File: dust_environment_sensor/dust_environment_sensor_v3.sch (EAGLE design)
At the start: 49 parts, among them IC2 ATMEGA644A, J1 3.6V Lithium C cell, J2 EXP, J3 XBEE_1-10SMT, J4 XBEE_11-20SMT, U1 TSL2560T, U2 LIS3DH, U3 SI7005, U4 TSL2560CL, U5 AMN41121, U6 L3GD20, U7 MCP1700-3.3V, X2 32.768KHz

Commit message: tiny DES3
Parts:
- removed C13, C15, C5: 100n, rcl:C-EUC0603
- removed C14: 10u, rcl:C-USC0603
- removed C7: 4.7u, rcl:C-USC0603
- removed J2: EXP, SparkFun-Connectors:AVR_SPI_PRG_6PTH
- removed JP4, JP5, JP6, JP7: M01PTH, SparkFun-Connectors:M01PTH
- removed R3: 15, resistor:R-US_R0603
- removed U3: SI7005, Cool_Electricity:SI7005
- removed U6: L3GD20, Cool_Electricity:L3GD20
- added EXP: M05X2SHD, SparkFun-Connectors:M05X2SHD
- C4: value 100u -> 100n; device SparkFun-Capacitors:CAP_POL1206-KIT -> rcl:C-EUC0603
- JP9: device SparkFun-Connectors:M05X2PTH -> SparkFun-Connectors:M05X2SHD
- U4: value TSL2560CL -> HTU21D; device Cool_Electricity:TSL2560CL -> Cool_Electricity:HTU21D
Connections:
- removed net N$1: C7.1, U3.CEXT
- removed net N$11: C5.1, R3.2, U3.VDD
- removed net N$2: C15.1, U6.CAP
- new net MOTE_ASSOCIATED: J4.ON/!SLEEP
- new net MOTE_CONNECT: J3.PWM0/RSSI
- new net MOTE_SLEEP: J3.DIO12
- new net MOTE_TCPSTATUS: J4.ASSOC/AD5/DIO5
- net EXP_CSN: now also EXP.9; no longer J2.5
- net EXP_MISO: now also EXP.5; no longer J2.1
- net EXP_MOSI: now also EXP.8; no longer J2.4
- net EXP_SCK: now also EXP.7; no longer J2.3
- net GND: now also C4.2, EXP.10, EXP.4; no longer C13.2, C14.2, C15.2, C4.-, C5.2, C7.2, J2.6, JP4.1, JP5.1, JP6.1, JP7.1, U3.GND@1, U3.GND@2, U3.GND@3, U3.GND@4, U3.PAD, U4.ADDR, U6.GND, U6.RES/GND@1, U6.RES/GND@2, U6.RES/GND@3, U6.RES/GND@4, U6.RES/GND@5
- net GYRO_INT2: no longer U6.DRDY/INT2
- net HUMID_CS: no longer U3.#CS
- net HUMID_VCC: no longer R3.1
- net I2C_SCL: now also EXP.2; no longer U3.SCL, U6.SCL/SPC
- net I2C_SDA: now also EXP.1; no longer U3.SDA, U6.SDA/SDI/SDO
- net LIGHT_INT: no longer U4.INT
- net MOTE_ASSOC: no longer J4.ASSOC/AD5/DIO5
- net MOTE_STATUS: no longer J4.ON/!SLEEP
- net VBATT: now also EXP.6; no longer C4.+, J2.2
- net VCC: now also C4.1, EXP.3; no longer C13.1, C14.1, U6.CS, U6.RES/VDD, U6.SDO/SA0, U6.VDD, U6.VDD_IO
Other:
- note added: "1: VCC 2: UART_TX 3: UART_RX 4: GPIO 8 / TRIGSLP 5: RESET 6: GPIO 5 / TRIGTCP / LED 7: GPIO 7 8: GPIO 9 9: GPIO 1 10: GND"
- note added: "20: SEN 2 19: GPIO 2 18: GPIO 3 17: SEN 5 16: UART_CTS 15: GPIO 6/ TCPSTATUS / LED 14: NC 13: GPIO4/ ASSOC / LED 12: UART_RTS 11: GPIO 14"
- note added: "Wifly Pinout"
- note removed: "I2C ADDRESS: 10000000"

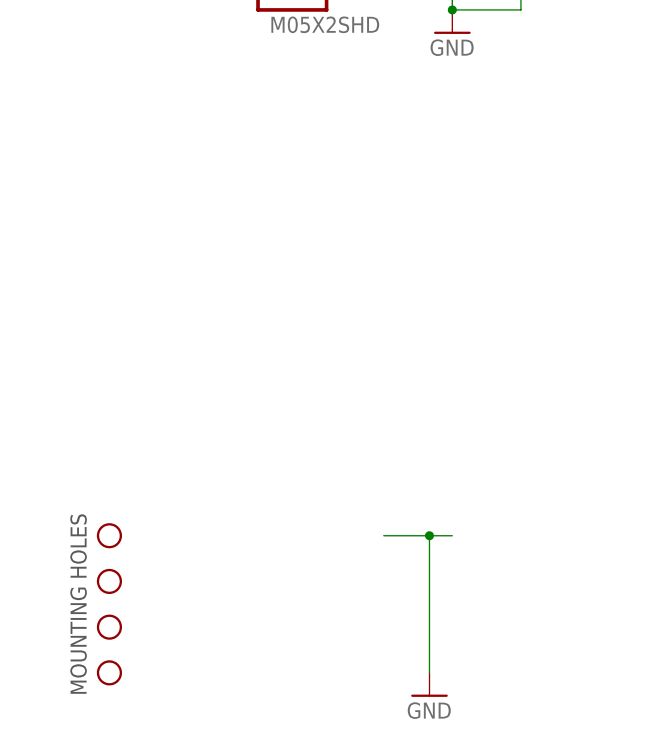
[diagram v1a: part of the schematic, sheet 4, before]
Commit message: schematic and placement done?
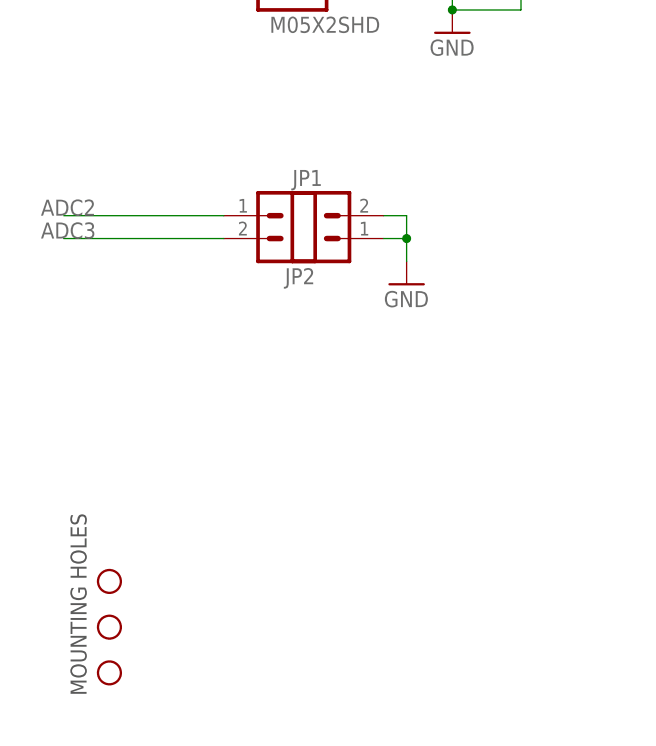
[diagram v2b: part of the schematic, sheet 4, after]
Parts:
- removed STANDOFF4: STAND-OFF, SparkFun-Electromechanical:STAND-OFF
- added JP1, JP2: (no value), SparkFun-Connectors:M02PTH
- J1: device Cool_Electricity:BX0036 -> Cool_Electricity:BX0036NH
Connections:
- removed net GYRO_INT2: IC2.(PCINT11/OC0A/AIN1)PB3
- removed net HUMID_CS: IC2.(PCINT2/ADC2)PA2
- removed net HUMID_VCC: IC2.(PCINT3/ADC3)PA3
- removed net MOTE_ASSOC: IC2.(PCINT9/CLKO/T1)PB1
- removed net MOTE_SLEEPN: IC2.(PCINT5/ADC5)PA5, J3.!DTR!/SLEEP_RQ/DIO8
- removed net MOTE_STATUS: IC2.(PCINT10/INT2/AIN0)PB2
- new net ADC2: IC2.(PCINT2/ADC2)PA2, JP2.1
- new net ADC3: IC2.(PCINT3/ADC3)PA3, JP2.2
- net GND: now also JP1.1, JP1.2
- net MOTE_ASSOCIATED: now also IC2.(PCINT11/OC0A/AIN1)PB3
- net MOTE_CONNECT: now also IC2.(PCINT9/CLKO/T1)PB1
- net MOTE_SLEEP: now also IC2.(PCINT5/ADC5)PA5
- net MOTE_TCPSTATUS: now also IC2.(PCINT10/INT2/AIN0)PB2
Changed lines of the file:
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@@
 <part name="GND2" library="supply1" deviceset="GND" device=""/>
 <part name="GND6" library="supply1" deviceset="GND" device=""/>
-<part name="J1" library="Cool_Electricity" deviceset="BX0036" device="" value="3.6V Lithium C cell"/>
+<part name="J1" library="Cool_Electricity" deviceset="BX0036" device="NH" value="3.6V Lithium C cell"/>
 <part name="GND7" library="supply1" deviceset="GND" device=""/>
 <part name="P+2" library="supply1" deviceset="VCC" device=""/>
@@
 <part name="STANDOFF2" library="SparkFun-Electromechanical" deviceset="STAND-OFF" device=""/>
 <part name="STANDOFF3" library="SparkFun-Electromechanical" deviceset="STAND-OFF" device=""/>
-<part name="STANDOFF4" library="SparkFun-Electromechanical" deviceset="STAND-OFF" device=""/>
-<part name="GND16" library="supply1" deviceset="GND" device=""/>
 <part name="GND17" library="SparkFun" deviceset="GND" device=""/>
 <part name="C8" library="rcl" deviceset="C-EU" device="C0603" value="100n"/>
@@
 <part name="GND13" library="supply1" deviceset="GND" device=""/>
 <part name="P+8" library="supply1" deviceset="VCC" device=""/>
+<part name="JP1" library="SparkFun-Connectors" deviceset="M02" device="PTH"/>
+<part name="JP2" library="SparkFun-Connectors" deviceset="M02" device="PTH"/>
+<part name="GND3" library="SparkFun" deviceset="GND" device=""/>
 </parts>
 <sheets>
@@
 <pinref part="IC2" gate="G$1" pin="(PCINT6/ADC6)PA6"/>
 <wire x1="119.38" y1="106.68" x2="160.02" y2="106.68" width="0.1524" layer="91"/>
-<label x="147.32" y="106.68" size="1.778" layer="95"/>
+<label x="142.24" y="106.68" size="1.778" layer="95"/>
 </segment>
 </net>
@@
 <wire x1="119.38" y1="38.1" x2="160.02" y2="38.1" width="0.1524" layer="91"/>
 <label x="134.62" y="38.1" size="1.778" layer="95"/>
-</segment>
-</net>
-<net name="MOTE_SLEEPN" class="0">
-<segment>
-<pinref part="IC2" gate="G$1" pin="(PCINT5/ADC5)PA5"/>
-<wire x1="119.38" y1="104.14" x2="160.02" y2="104.14" width="0.1524" layer="91"/>
-<label x="142.24" y="104.14" size="1.778" layer="95"/>
 </segment>
 </net>
@@
 </segment>
 </net>
-<net name="GYRO_INT2" class="0">
-<segment>
-<pinref part="IC2" gate="G$1" pin="(PCINT11/OC0A/AIN1)PB3"/>
-<wire x1="119.38" y1="76.2" x2="154.94" y2="76.2" width="0.1524" layer="91"/>
-<label x="144.78" y="76.2" size="1.778" layer="95"/>
-</segment>
-</net>
-<net name="HUMID_CS" class="0">
-<segment>
-<pinref part="IC2" gate="G$1" pin="(PCINT2/ADC2)PA2"/>
-<wire x1="119.38" y1="96.52" x2="157.48" y2="96.52" width="0.1524" layer="91"/>
-<label x="137.16" y="96.52" size="1.778" layer="95"/>
-</segment>
-</net>
-<net name="HUMID_VCC" class="0">
-<segment>
-<pinref part="IC2" gate="G$1" pin="(PCINT3/ADC3)PA3"/>
-<wire x1="119.38" y1="99.06" x2="160.02" y2="99.06" width="0.1524" layer="91"/>
-<label x="139.7" y="99.06" size="1.778" layer="95"/>
-</segment>
-</net>
-<net name="MOTE_STATUS" class="0">
+<net name="MOTE_TCPSTATUS" class="0">
 <segment>
 <pinref part="IC2" gate="G$1" pin="(PCINT10/INT2/AIN0)PB2"/>
@@
 </segment>
 </net>
-<net name="MOTE_ASSOC" class="0">
+<net name="MOTE_TX_CTSN" class="0">
+<segment>
+<pinref part="IC2" gate="G$1" pin="(PCINT8/XCK0/T0)PB0"/>
+<wire x1="119.38" y1="68.58" x2="152.4" y2="68.58" width="0.1524" layer="91"/>
+<label x="139.7" y="68.58" size="1.778" layer="95"/>
+</segment>
+</net>
+<net name="MOTE_CONNECT" class="0">
 <segment>
 <pinref part="IC2" gate="G$1" pin="(PCINT9/CLKO/T1)PB1"/>
@@
 </segment>
 </net>
-<net name="MOTE_TX_CTSN" class="0">
-<segment>
-<pinref part="IC2" gate="G$1" pin="(PCINT8/XCK0/T0)PB0"/>
-<wire x1="119.38" y1="68.58" x2="152.4" y2="68.58" width="0.1524" layer="91"/>
-<label x="139.7" y="68.58" size="1.778" layer="95"/>
+<net name="ADC2" class="0">
+<segment>
+<pinref part="IC2" gate="G$1" pin="(PCINT2/ADC2)PA2"/>
+<wire x1="119.38" y1="96.52" x2="157.48" y2="96.52" width="0.1524" layer="91"/>
+<label x="142.24" y="96.52" size="1.778" layer="95"/>
+</segment>
+</net>
+<net name="MOTE_ASSOCIATED" class="0">
+<segment>
+<pinref part="IC2" gate="G$1" pin="(PCINT11/OC0A/AIN1)PB3"/>
+<wire x1="119.38" y1="76.2" x2="157.48" y2="76.2" width="0.1524" layer="91"/>
+<label x="139.7" y="76.2" size="1.778" layer="95"/>
+</segment>
+</net>
+<net name="MOTE_SLEEP" class="0">
+<segment>
+<pinref part="IC2" gate="G$1" pin="(PCINT5/ADC5)PA5"/>
+<wire x1="119.38" y1="104.14" x2="160.02" y2="104.14" width="0.1524" layer="91"/>
+<label x="142.24" y="104.14" size="1.778" layer="95"/>
+</segment>
+</net>
+<net name="ADC3" class="0">
+<segment>
+<pinref part="IC2" gate="G$1" pin="(PCINT3/ADC3)PA3"/>
+<wire x1="119.38" y1="99.06" x2="157.48" y2="99.06" width="0.1524" layer="91"/>
+<label x="142.24" y="99.06" size="1.778" layer="95"/>
 </segment>
 </net>
@@
 </segment>
 </net>
-<net name="MOTE_SLEEPN" class="0">
-<segment>
-<pinref part="J3" gate="G$1" pin="!DTR!/SLEEP_RQ/DIO8"/>
-<wire x1="43.18" y1="20.32" x2="15.24" y2="20.32" width="0.1524" layer="91"/>
-<label x="15.24" y="20.32" size="1.778" layer="95"/>
-</segment>
-</net>
 <net name="MOTE_RESETN" class="0">
 <segment>
@@
 <instance part="STANDOFF2" gate="G$1" x="10.16" y="12.7" rot="R90"/>
 <instance part="STANDOFF3" gate="G$1" x="10.16" y="17.78" rot="R90"/>
-<instance part="STANDOFF4" gate="G$1" x="10.16" y="22.86" rot="R90"/>
-<instance part="GND16" gate="1" x="45.72" y="5.08"/>
 <instance part="JP8" gate="G$1" x="116.84" y="68.58" rot="R180"/>
 <instance part="GND21" gate="1" x="104.14" y="78.74" rot="R180"/>
@@
 <instance part="EXP" gate="G$1" x="30.48" y="88.9"/>
 <instance part="GND10" gate="1" x="48.26" y="78.74"/>
+<instance part="JP1" gate="G$1" x="33.02" y="55.88"/>
+<instance part="JP2" gate="G$1" x="30.48" y="58.42" rot="R180"/>
+<instance part="GND3" gate="1" x="43.18" y="50.8"/>
 </instances>
 <busses>
@@
 <nets>
 <net name="GND" class="0">
-<segment>
-<wire x1="40.64" y1="22.86" x2="45.72" y2="22.86" width="0.1524" layer="91"/>
-<pinref part="GND16" gate="1" pin="GND"/>
-<wire x1="45.72" y1="22.86" x2="48.26" y2="22.86" width="0.1524" layer="91"/>
-<wire x1="45.72" y1="22.86" x2="45.72" y2="7.62" width="0.1524" layer="91"/>
-<junction x="45.72" y="22.86"/>
-</segment>
 <segment>
 <pinref part="JP8" gate="G$1" pin="CTS"/>
@@
 <junction x="48.26" y="81.28"/>
 </segment>
+<segment>
+<pinref part="JP1" gate="G$1" pin="1"/>
+<pinref part="GND3" gate="1" pin="GND"/>
+<wire x1="40.64" y1="55.88" x2="43.18" y2="55.88" width="0.1524" layer="91"/>
+<wire x1="43.18" y1="55.88" x2="43.18" y2="53.34" width="0.1524" layer="91"/>
+<pinref part="JP1" gate="G$1" pin="2"/>
+<wire x1="40.64" y1="58.42" x2="43.18" y2="58.42" width="0.1524" layer="91"/>
+<wire x1="43.18" y1="58.42" x2="43.18" y2="55.88" width="0.1524" layer="91"/>
+<junction x="43.18" y="55.88"/>
+</segment>
 </net>
 <net name="VBATT" class="0">
@@
 </segment>
 </net>
+<net name="ADC2" class="0">
+<segment>
+<pinref part="JP2" gate="G$1" pin="1"/>
+<wire x1="22.86" y1="58.42" x2="5.08" y2="58.42" width="0.1524" layer="91"/>
+<label x="2.54" y="58.42" size="1.778" layer="95"/>
+</segment>
+</net>
+<net name="ADC3" class="0">
+<segment>
+<pinref part="JP2" gate="G$1" pin="2"/>
+<wire x1="22.86" y1="55.88" x2="5.08" y2="55.88" width="0.1524" layer="91"/>
+<label x="2.54" y="55.88" size="1.778" layer="95"/>
+</segment>
+</net>
